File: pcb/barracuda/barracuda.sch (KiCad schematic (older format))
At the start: 69 parts, among them SW1 SW_PUSH, SW10 SW_PUSH, SW11 SW_PUSH, SW12 SW_PUSH, SW13 SW_PUSH, SW14 SW_PUSH, SW15 SW_PUSH, SW16 SW_PUSH, SW17 SW_PUSH, SW18 SW_PUSH, SW19 SW_PUSH, SW2 SW_PUSH, SW20 SW_PUSH, SW21 SW_PUSH, SW22 SW_PUSH, SW23 SW_PUSH, SW24 SW_PUSH, SW25 SW_PUSH, SW26 SW_PUSH, SW27 SW_PUSH, SW28 SW_PUSH, SW29 SW_PUSH, SW3 SW_PUSH, SW30 SW_PUSH, SW31 SW_PUSH, SW32 SW_PUSH, SW33 SW_PUSH, SW4 SW_PUSH, SW5 SW_PUSH, SW6 SW_PUSH, SW7 SW_PUSH, SW8 SW_PUSH, SW9 SW_PUSH, U1 ProMicro

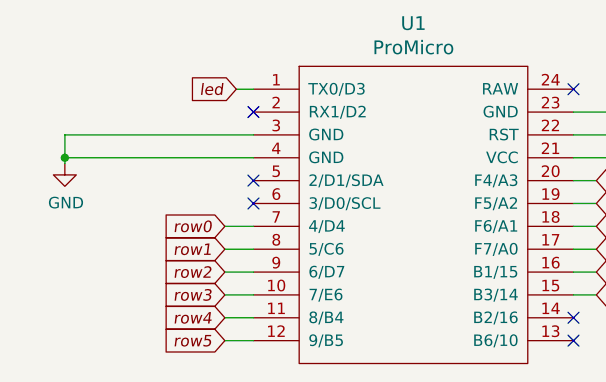
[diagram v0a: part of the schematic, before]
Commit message: PCB almost done
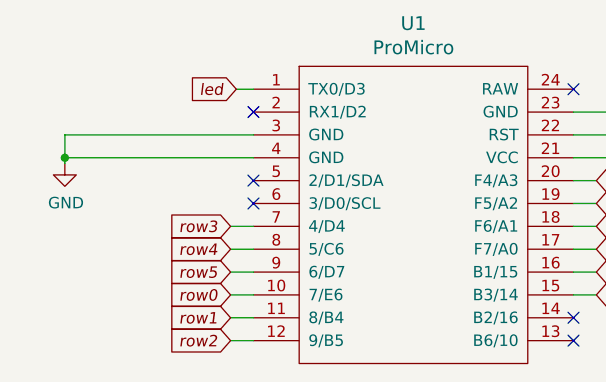
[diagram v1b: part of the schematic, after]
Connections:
- net row0: now also U1.10 (7/E6); no longer U1.7 (4/D4)
- net row1: now also U1.11 (8/B4); no longer U1.8 (5/C6)
- net row2: now also U1.12 (9/B5); no longer U1.9 (6/D7)
- net row3: now also U1.7 (4/D4); no longer U1.10 (7/E6)
- net row4: now also U1.8 (5/C6); no longer U1.11 (8/B4)
- net row5: now also U1.9 (6/D7); no longer U1.12 (9/B5)
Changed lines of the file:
@@
 	5125 5200 6000 5200
 Connection ~ 5125 5200
-Text GLabel 1300 6975 0    50   Input Italic 0
+Text GLabel 1325 7275 0    50   Input Italic 0
 row0
-Text GLabel 1300 7075 0    50   Input Italic 0
+Text GLabel 1325 7375 0    50   Input Italic 0
 row1
-Text GLabel 1300 7175 0    50   Input Italic 0
+Text GLabel 1325 7475 0    50   Input Italic 0
 row2
-Text GLabel 1300 7275 0    50   Input Italic 0
+Text GLabel 1325 6975 0    50   Input Italic 0
 row3
-Text GLabel 1300 7375 0    50   Input Italic 0
+Text GLabel 1325 7075 0    50   Input Italic 0
 row4
-Text GLabel 1300 7475 0    50   Input Italic 0
+Text GLabel 1325 7175 0    50   Input Italic 0
 row5
 Text GLabel 2925 6775 2    50   Input Italic 0
@@
 Wire Wire Line
 	2825 7275 2925 7275
-Wire Wire Line
-	1300 6975 1425 6975
-Wire Wire Line
-	1300 7075 1425 7075
-Wire Wire Line
-	1300 7175 1425 7175
-Wire Wire Line
-	1300 7375 1425 7375
-Wire Wire Line
-	1300 7475 1425 7475
-Wire Wire Line
-	1300 7275 1425 7275
 NoConn ~ 2825 6375
 NoConn ~ 2825 7475
@@
 Wire Wire Line
 	2500 5200 4250 5200
+Wire Wire Line
+	1325 7275 1425 7275
+Wire Wire Line
+	1325 7375 1425 7375
+Wire Wire Line
+	1325 7475 1425 7475
+Wire Wire Line
+	1325 6975 1425 6975
+Wire Wire Line
+	1325 7075 1425 7075
+Wire Wire Line
+	1325 7175 1425 7175
 $EndSCHEMATC
